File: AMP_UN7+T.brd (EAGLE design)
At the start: 80 x 40 mm, 54 parts

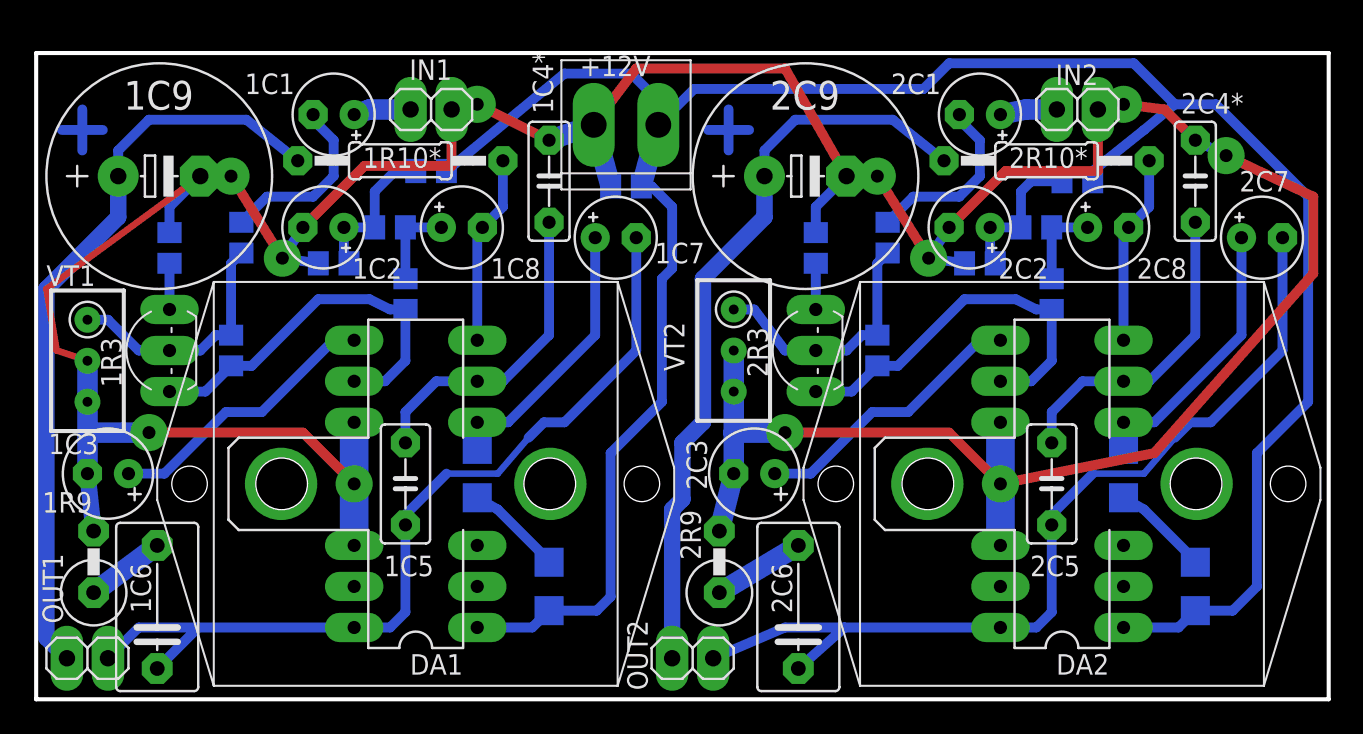
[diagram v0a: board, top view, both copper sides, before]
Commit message: 5
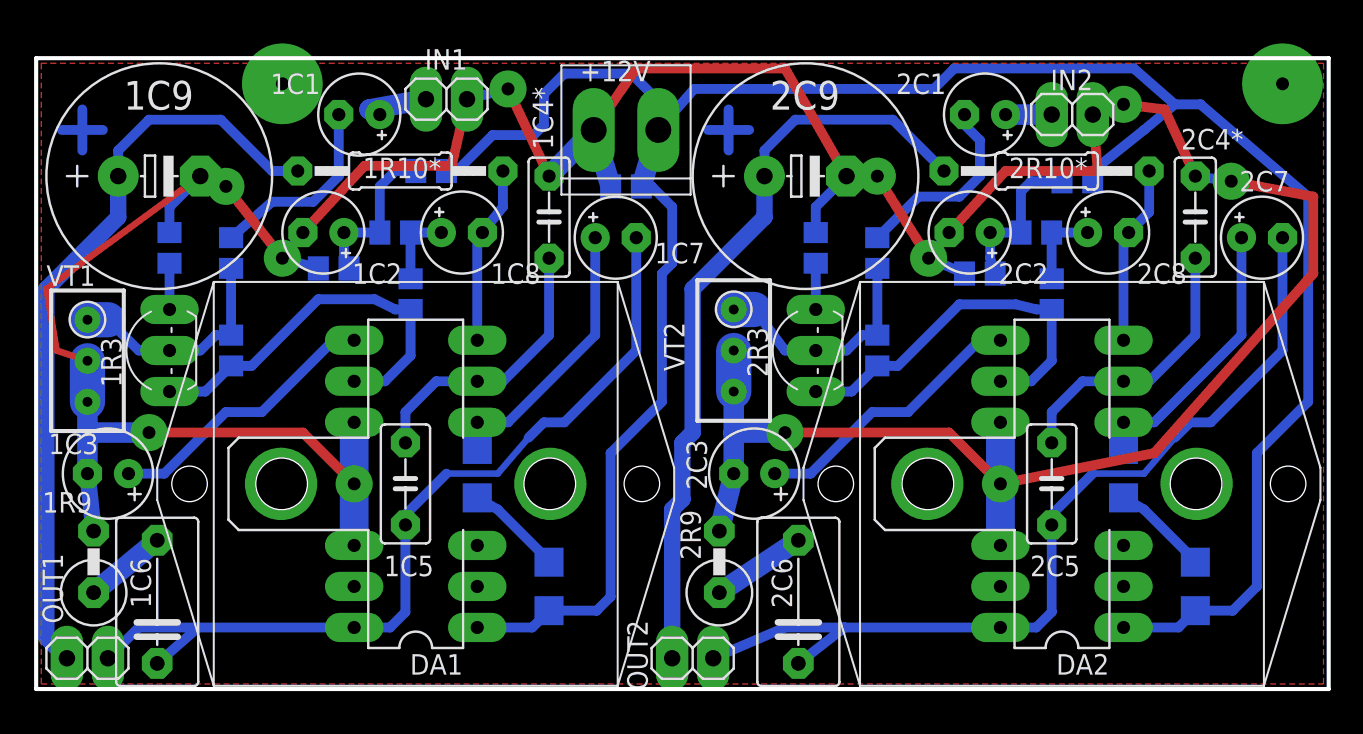
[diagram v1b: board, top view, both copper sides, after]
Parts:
- moved 1C4* 2.22 mm to (-31.1, 114.3)
- moved 2C4* 2.22 mm to (8.89, 114.3)
- moved 1C1 1.59 mm to (-42.9, 120.7)
- moved 2R1 1.14 mm to (-10.8, 112.1)
- moved 1R1 1.14 mm to (-50.8, 112.1)
- moved IN1 1.14 mm to (-37.5, 121.6)
- moved 1R10* 0.64 mm to (-40.3, 117.2)
- moved 2R10* 0.64 mm to (-0.32, 117.2)
- moved 2C10 0.63 mm to (-4.45, 110.8)
- moved 1R4 0.45 mm to (-40.6, 113.3)
- moved IN2 0.45 mm to (1.27, 120.7)
- moved 1C2 0.32 mm to (-45.1, 113.3)
- moved 1C8 0.32 mm to (-36.5, 113.3)
- moved 2C2 0.32 mm to (-5.08, 113.3)
- moved 2C8 0.32 mm to (3.49, 113.3)
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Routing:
- net GND: track 231.6 -> 236.3 mm
- net N$24: track 19.8 -> 17.5 mm
- net N$11: track 19.8 -> 17.5 mm
- net N$3: track 15.4 -> 14.2 mm
- net N$19: track 11.2 -> 12.4 mm
- net +12V: track 145.8 -> 146.9 mm
- net N$18: track 15.9 -> 15.0 mm
- net N$4: track 11.2 -> 12.0 mm
- net IN1: track 3.54 -> 4.26 mm
- net IN2: track 3.52 -> 2.86 mm
- net N$5: track 5.40 -> 4.77 mm
- net N$21: track 9.29 -> 9.84 mm
- net N$13: track 11.8 -> 11.2 mm
- added copper zone on layer 1, net GND
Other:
- board size 80 x 40 mm -> 80 x 39.1 mm

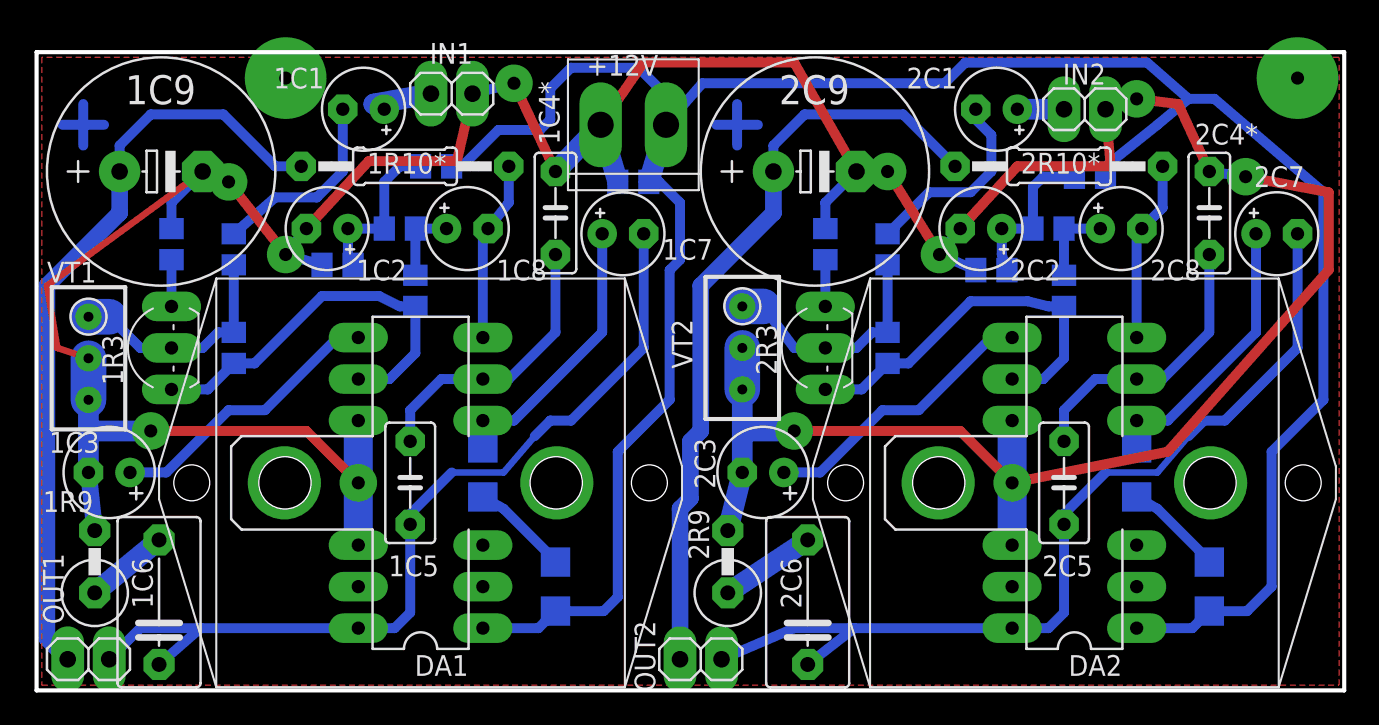
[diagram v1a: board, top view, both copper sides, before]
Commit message: .
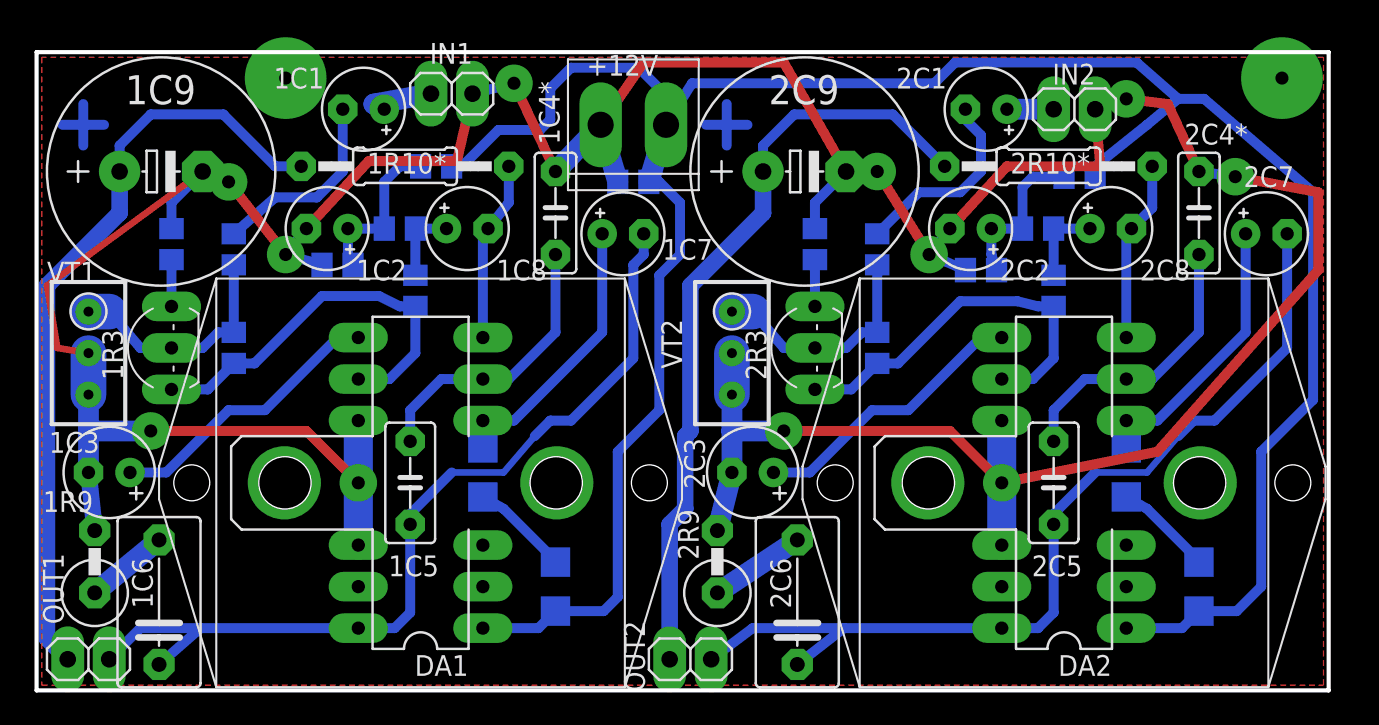
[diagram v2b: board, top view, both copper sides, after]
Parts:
- moved 2R3 0.71 mm to (-20.3, 105.7)
- moved 2C3 0.64 mm to (-19.1, 98.4)
- moved 2C6 0.64 mm to (-16.3, 90.5)
- moved VT2 0.64 mm to (-16.5, 106.0)
- moved 2C8 0.64 mm to (2.86, 113.3)
- moved 2R8' 0.64 mm to (3.81, 98.4)
- moved 2C5 0.64 mm to (-0.64, 97.8)
- moved 2R10* 0.64 mm to (-0.95, 117.2)
- moved 2R5 0.64 mm to (-0.64, 109.5)
- moved DA2 0.64 mm to (0.00, 97.8)
- moved HEATSINK2 0.64 mm to (0.00, 97.8)
- moved IN2 0.64 mm to (0.64, 120.7)
- moved 2R4 0.63 mm to (-1.59, 113.3)
- moved 2R7 0.63 mm to (0.95, 116.5)
- moved 2C1 0.63 mm to (-4.76, 120.7)
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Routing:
- net GND: track 236.3 -> 235.5 mm
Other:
- board size 80 x 39.1 mm -> 79.1 x 39.1 mm

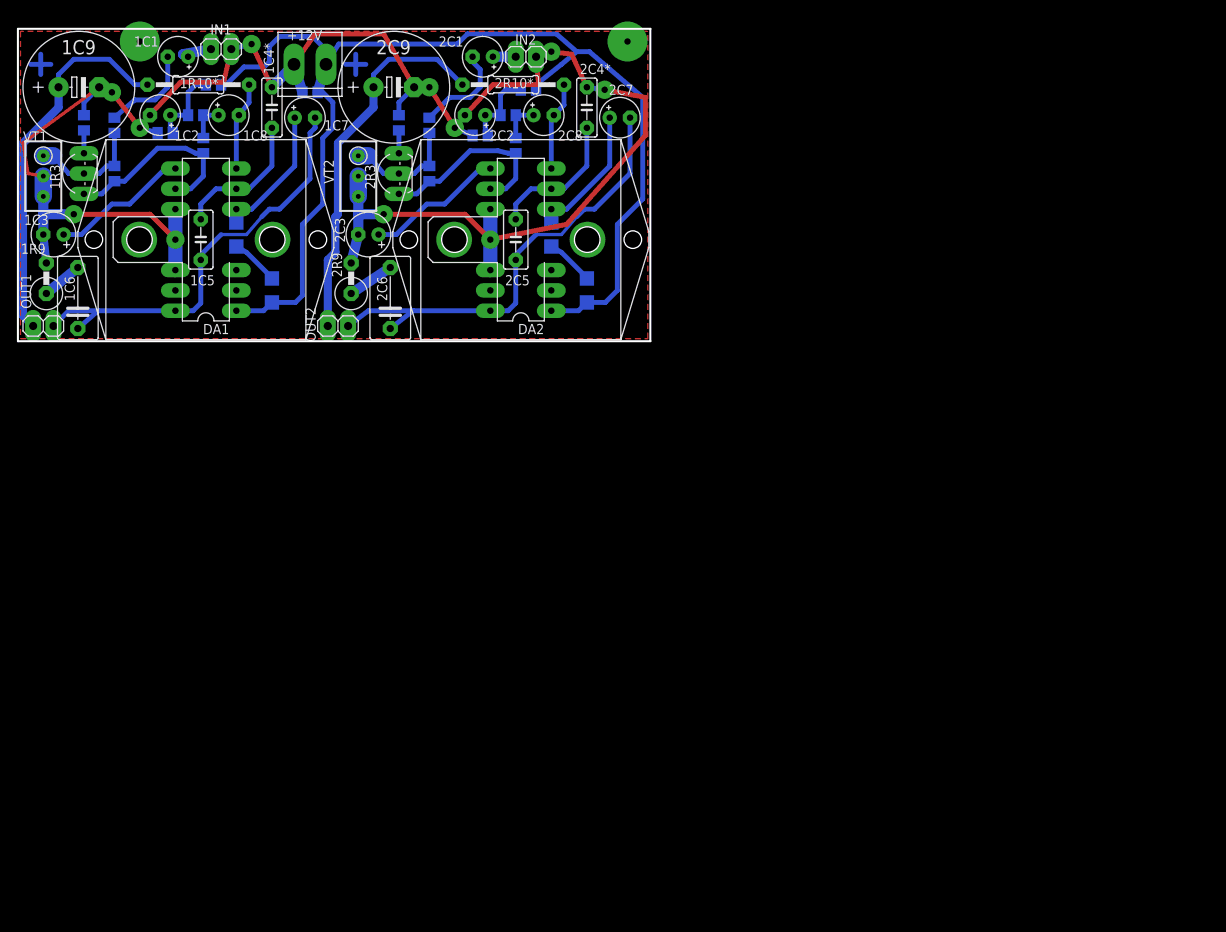
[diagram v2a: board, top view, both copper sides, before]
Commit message: 6
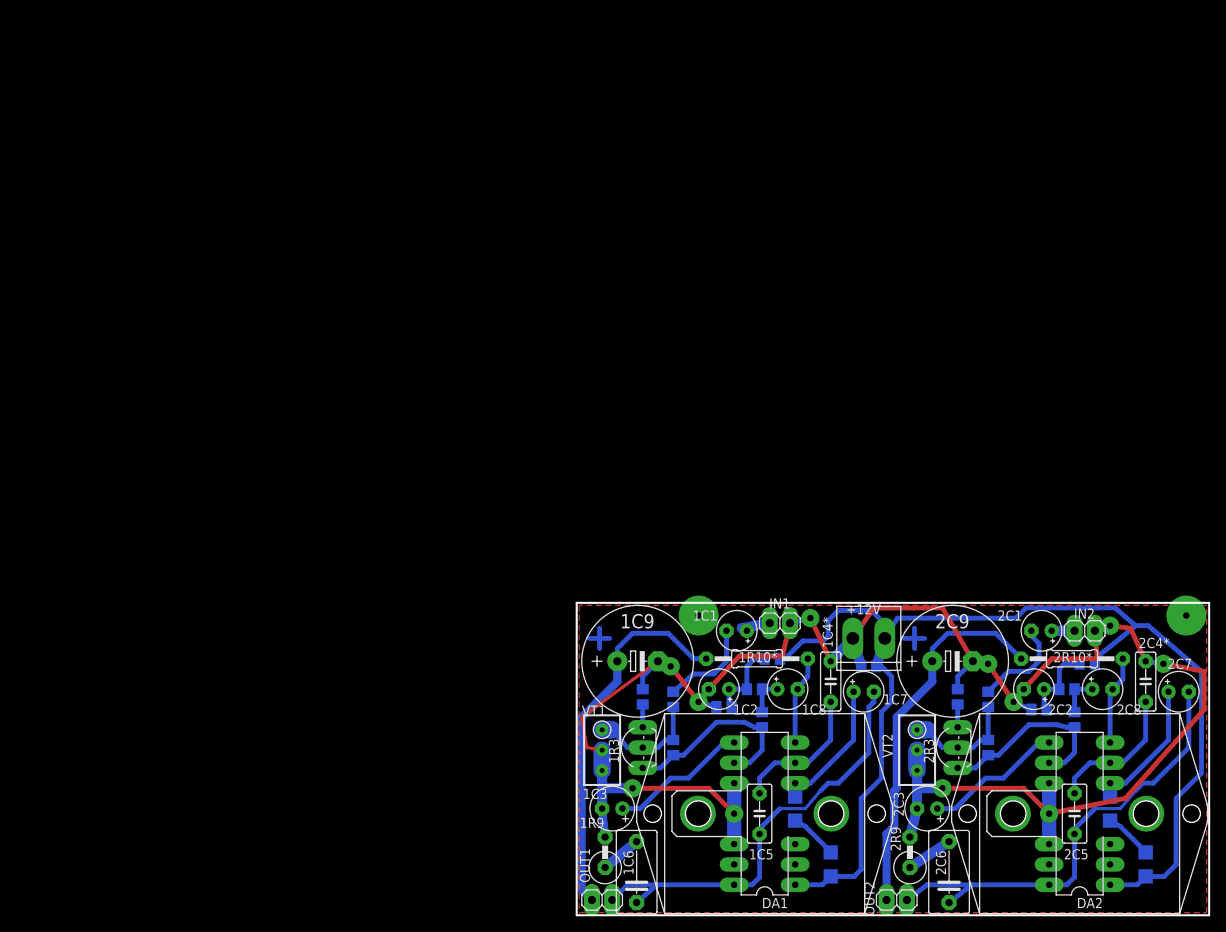
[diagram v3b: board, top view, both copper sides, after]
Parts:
- moved 2C1 100.1 mm to (65.1, 48.9)
- moved 2C2 100.1 mm to (64.1, 41.6)
- moved 2C4* 100.1 mm to (78.1, 42.5)
- moved 2C5 100.1 mm to (69.2, 26.0)
- moved 2C6 100.1 mm to (53.5, 18.7)
- moved 2R4 100.1 mm to (68.3, 41.6)
- moved 2R5 100.1 mm to (69.2, 37.8)
- moved 2R8 100.1 mm to (78.1, 19.7)
- moved VT1 100.1 mm to (14.0, 34.3)
- moved VT2 100.1 mm to (53.3, 34.3)
- moved +12V 100.1 mm to (43.5, 47.9)
- moved 1C1 100.1 mm to (27.0, 48.9)
- moved 1C10 100.1 mm to (25.4, 39.4)
- moved 1C2 100.1 mm to (24.8, 41.6)
- moved 1C3 100.1 mm to (11.4, 26.7)
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
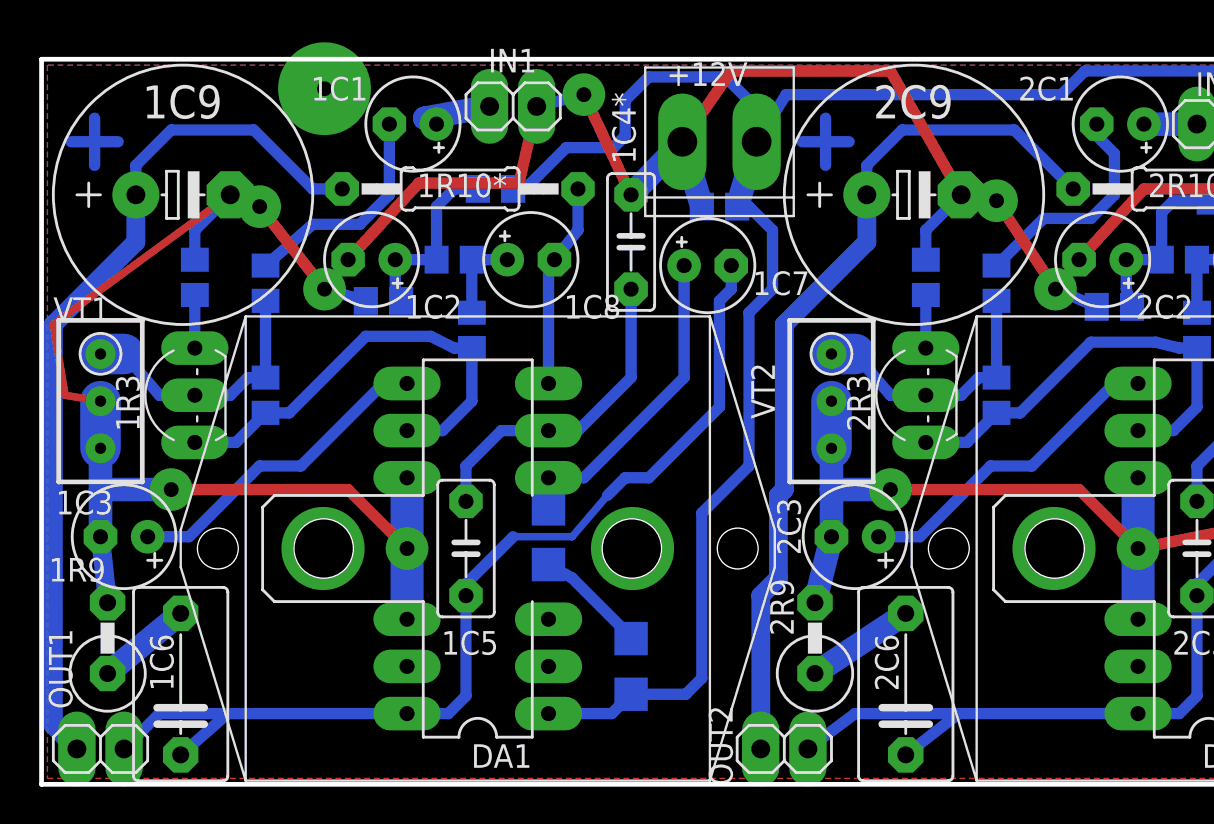
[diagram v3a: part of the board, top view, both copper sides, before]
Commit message: 7
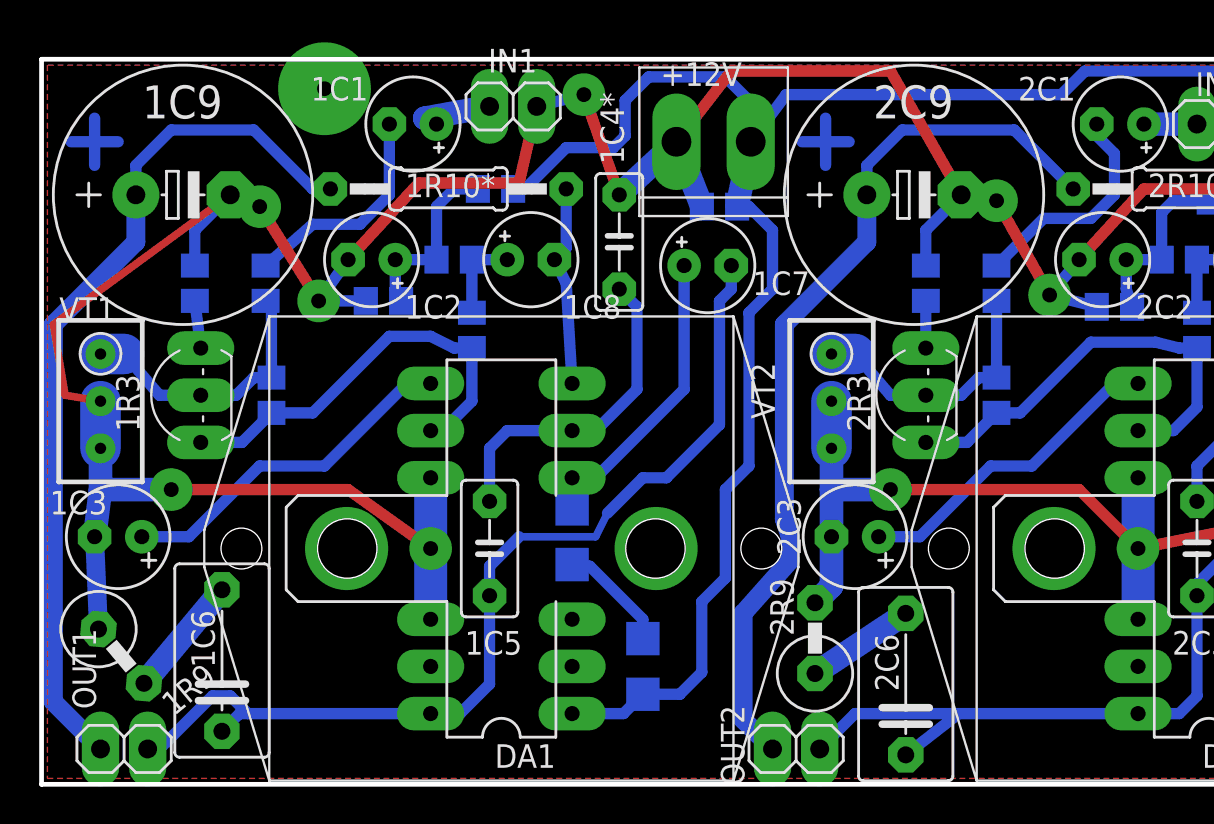
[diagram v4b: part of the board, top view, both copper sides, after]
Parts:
- moved 1C6 2.56 mm to (16.7, 20.0)
- moved 1R9 2.39 mm to (11.7, 19.7), turned to 310 degrees
- moved 1R8' 1.27 mm to (35.6, 26.7)
- moved 1C5 1.27 mm to (31.1, 26.0)
- moved DA1 1.27 mm to (31.8, 26.0)
- moved HEATSINK1 1.27 mm to (31.8, 26.0)
- moved OUT1 1.27 mm to (11.4, 15.2)
- moved 1R10* 0.64 mm to (28.9, 45.4)
- moved 1C4* 0.63 mm to (38.1, 42.5)
- moved 1R8 0.63 mm to (39.4, 19.7)
- moved OUT2 0.63 mm to (47.6, 15.2)
- moved +12V 0.32 mm to (43.2, 47.9)
- moved 1R6 0.32 mm to (15.2, 40.3)
- moved 2R6 0.32 mm to (54.6, 40.3)
- moved 1C3 0.32 mm to (11.1, 26.7)
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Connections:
- net GND: now also 1R9.1; no longer 1R9.2
- net N$12: now also 1R9.2; no longer 1R9.1
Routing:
- net GND: track 235.3 -> 240.9 mm
- net N$8: track 17.4 -> 19.0 mm
- net N$1: track 24.4 -> 22.9 mm
- net N$12: track 5.10 -> 6.56 mm
- net +12V: track 146.5 -> 145.2 mm
- net OUT1+: track 54.6 -> 53.4 mm
- net OUT2-: track 47.0 -> 48.2 mm
- net N$9: track 17.2 -> 16.3 mm
